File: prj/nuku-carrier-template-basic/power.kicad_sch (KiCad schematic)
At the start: 11 parts, among them U1 AP61302

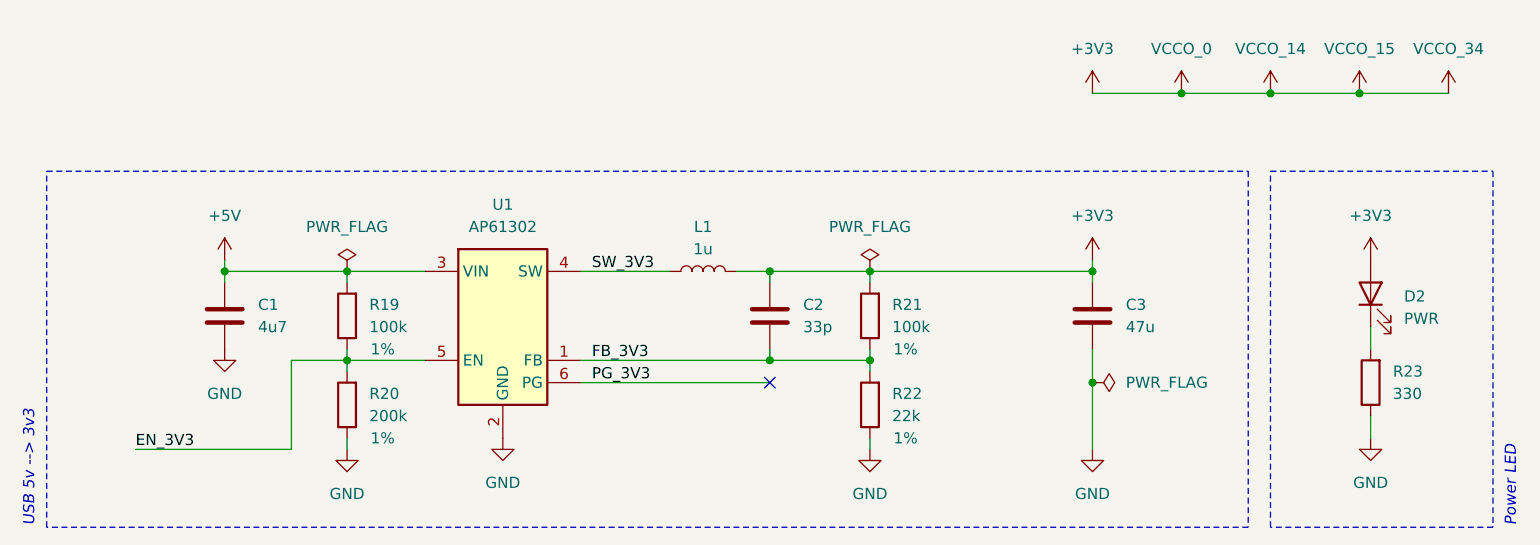
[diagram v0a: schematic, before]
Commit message: Route template.basic
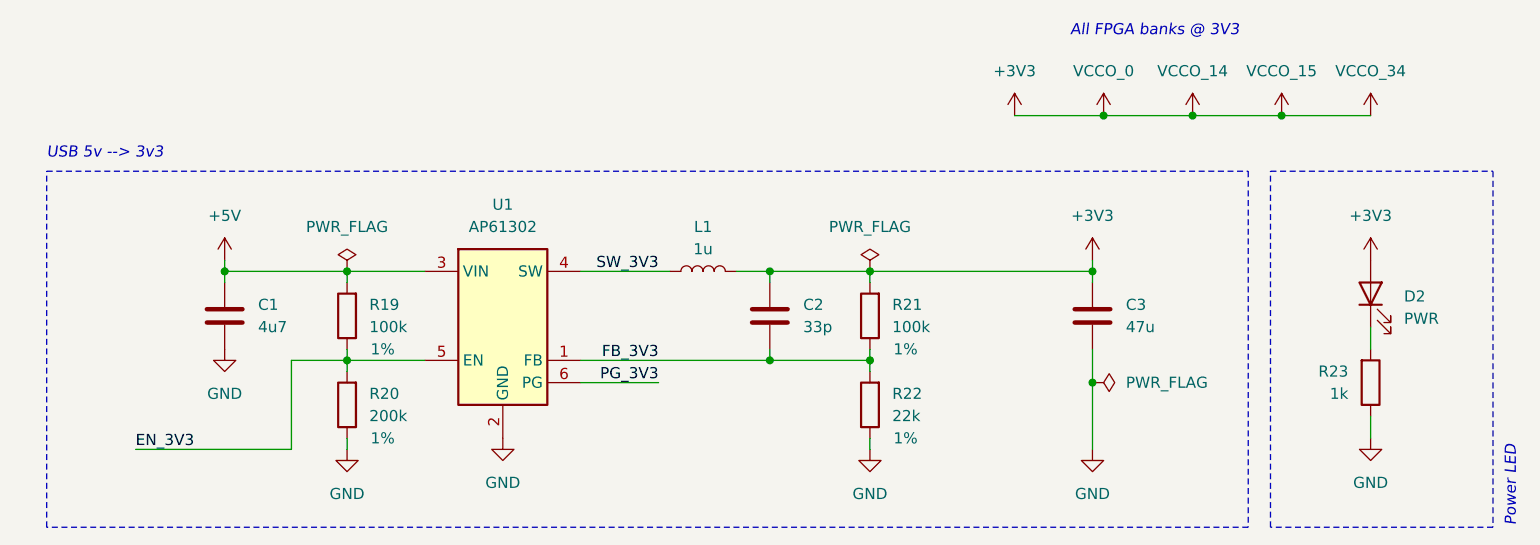
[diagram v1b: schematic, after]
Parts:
- R23: value 330 -> 1k; LCSC C25104 -> C11702
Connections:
- no-connect marks 1 -> 0
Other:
- note added: "All FPGA banks @ 3V3"
